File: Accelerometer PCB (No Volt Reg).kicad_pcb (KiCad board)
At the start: 2 copper layers, 77 x 55 mm, 21 parts, among them J1 S2B-PH-SM4-TB_LF__SN_, J2 M20-8770442, J3 MolexMicroSD, SW1 SW_Push, SW2 SW_Push, U1 Swan v3.0, U2 Sysrox Accelerometer, U3 Adafruit DS3231 RTC

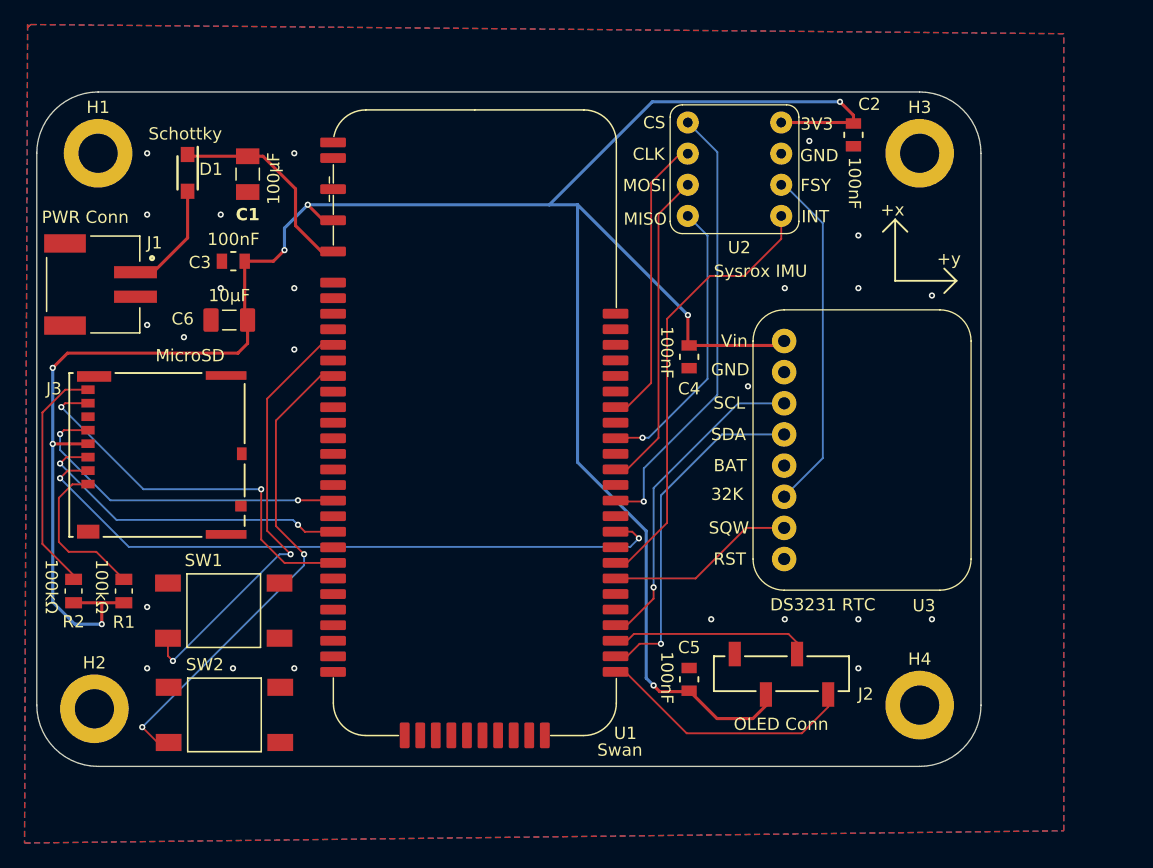
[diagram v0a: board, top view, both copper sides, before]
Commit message: Add files via upload
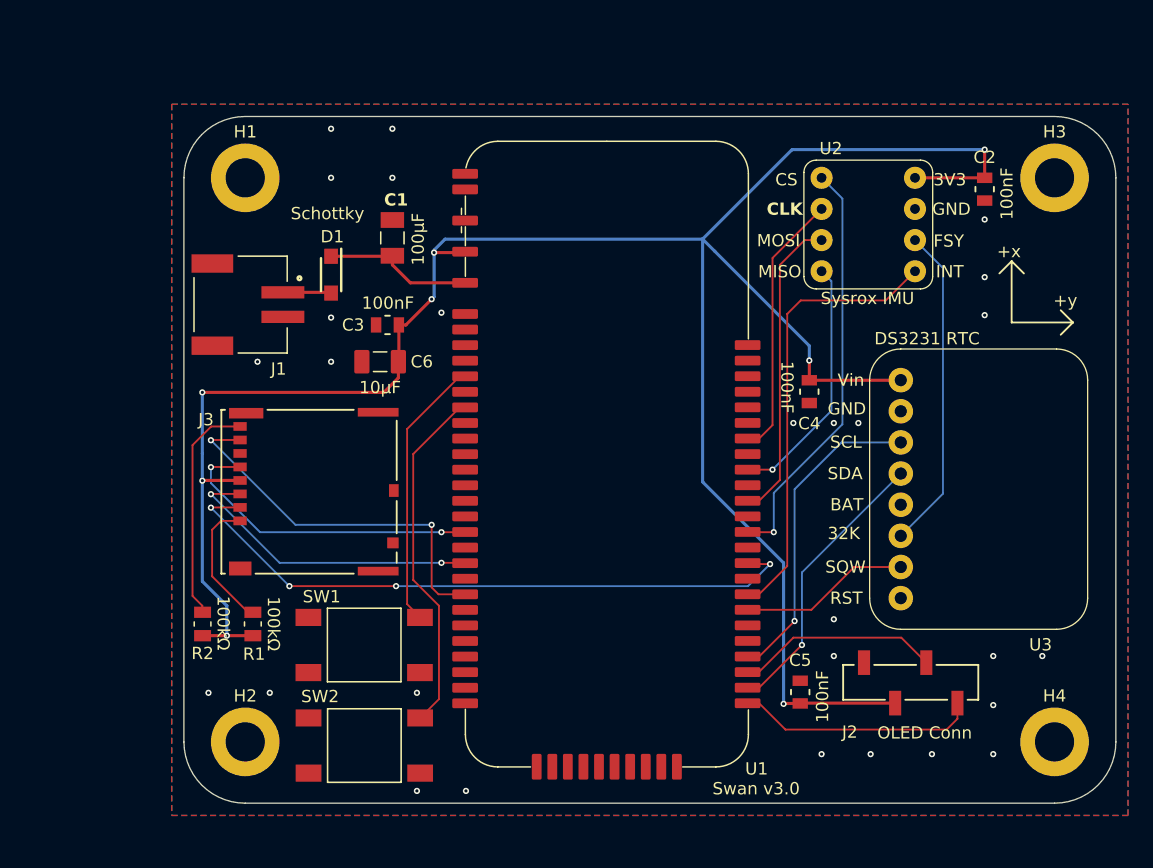
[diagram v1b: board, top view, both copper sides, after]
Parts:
- J1: value S2B-PH-SM4-TB_LF__SN_ -> Power Connector
- R1, R2: value 100k -> 100kΩ
- moved U2 19.8 mm to (170.9, 82.1), turned to 0 degrees
- moved D1 14.3 mm to (126.0, 80.9)
- moved C3 13.6 mm to (130.6, 85.0)
- moved C1 12.9 mm to (131.0, 77.9), turned to 90 degrees
- moved C6 12.8 mm to (130.0, 88.0)
- moved J3 12.8 mm to (124.2, 98.6)
- moved H2 12.6 mm to (119.0, 119.0)
- moved H1 12.2 mm to (119.0, 73.0)
- moved J1 12.1 mm to (122.1, 83.3)
- moved SW1 11.8 mm to (128.7, 111.1), turned to 180 degrees
- moved SW2 11.7 mm to (128.7, 119.3), turned to 180 degrees
- moved C2 11.6 mm to (179.3, 73.9)
- moved H4 11.4 mm to (185.0, 119.0)
- moved H3 11.2 mm to (185.0, 73.0)
- moved U1 11.1 mm to (128.2, 64.5)
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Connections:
- net Net-(D1-K) renamed Input Power
- net Net-(J2-SCL) renamed /OLED Serial Clock
- net Net-(J2-SDA) renamed /OLED Serial Data
- net Net-(J3-CD/DAT3) renamed /MicroSD Card Detect
- net Net-(J3-CLK) renamed /MicroSD Clock Line
- net Net-(J3-CMD) renamed /MicroSD MOSI
- net Net-(J3-DA0) renamed /MicroSD MISO
- net Net-(U1-A1) renamed /Switch 1 I/O
- net Net-(U1-A2) renamed /Switch 2 I/O
- net Net-(U1-D10) renamed /IMU Chip Select
- net Net-(U1-D11) renamed /IMU MOSI
- net Net-(U1-D12) renamed /IMU MISO
- net Net-(U1-D13) renamed /IMU Serial Clock
- net Net-(U1-D6) renamed /IMU Interrupt
- net Net-(U1-D8) renamed /RTC Square Wave
- net Net-(U1-SCL) renamed /RTC Clock Line
- net Net-(U1-SDA) renamed /RTC Data Line
- net Net-(U2-FSY) renamed /32kHz Frame Sync
- C2 pad 2: Net-(J2-VCC) -> +3.3V
- C3 pad 1: Net-(J2-VCC) -> +3.3V
- C4 pad 1: Net-(J2-VCC) -> +3.3V
- C5 pad 1: Net-(J2-VCC) -> +3.3V
- C6 pad 2: Net-(J2-VCC) -> +3.3V
- J2 pad 3: Net-(J2-VCC) -> +3.3V
- J3 pad 4: Net-(J2-VCC) -> +3.3V
- R1 pad 1: Net-(J3-DAT2) -> +3.3V
- R1 pad 2: Net-(J2-VCC) -> Net-(J3-DAT2)
- R2 pad 2: Net-(J2-VCC) -> +3.3V
- U1 pad 2: Net-(J2-VCC) -> +3.3V
- U2 pad 1: Net-(J2-VCC) -> +3.3V
- U3 pad 1: Net-(J2-VCC) -> +3.3V
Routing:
- net Net-(J2-VCC): track 200.6 -> 0.00 mm, vias 8 -> 0
- net +3.3V: track 0.00 -> 187.4 mm, vias 0 -> 8
- net /Switch 1 I/O: track 35.8 -> 22.3 mm, vias 2 -> 0
- net /Switch 2 I/O: track 40.2 -> 28.8 mm, vias 2 -> 0
- net Net-(D1-A): track 9.21 -> 3.95 mm
- net /RTC Data Line: track 27.4 -> 22.3 mm
- net Input Power: track 16.8 -> 12.2 mm
- net /IMU MISO: track 22.5 -> 19.6 mm
- net /IMU Chip Select: track 35.8 -> 33.1 mm
- net /IMU Serial Clock: track 23.1 -> 20.8 mm
- net Net-(J3-DAT2): track 13.0 -> 10.9 mm
- net /32kHz Frame Sync: track 28.3 -> 26.5 mm
- net /OLED Serial Data: track 20.5 -> 18.7 mm
- net /MicroSD Clock Line: track 27.6 -> 26.0 mm
- net /MicroSD MOSI: track 27.0 -> 25.4 mm
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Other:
- board size 77 x 55 mm -> 76 x 56 mm
- board text added: "Swan v3.0"
- board text removed: "MicroSD"
- board text removed: "PWR Conn"
- board text removed: "Swan"
- board text removed: "Sysrox IMU"
